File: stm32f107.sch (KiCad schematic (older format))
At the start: 12 parts, among them U5 STM32F107RCTx, Y2 Crystal

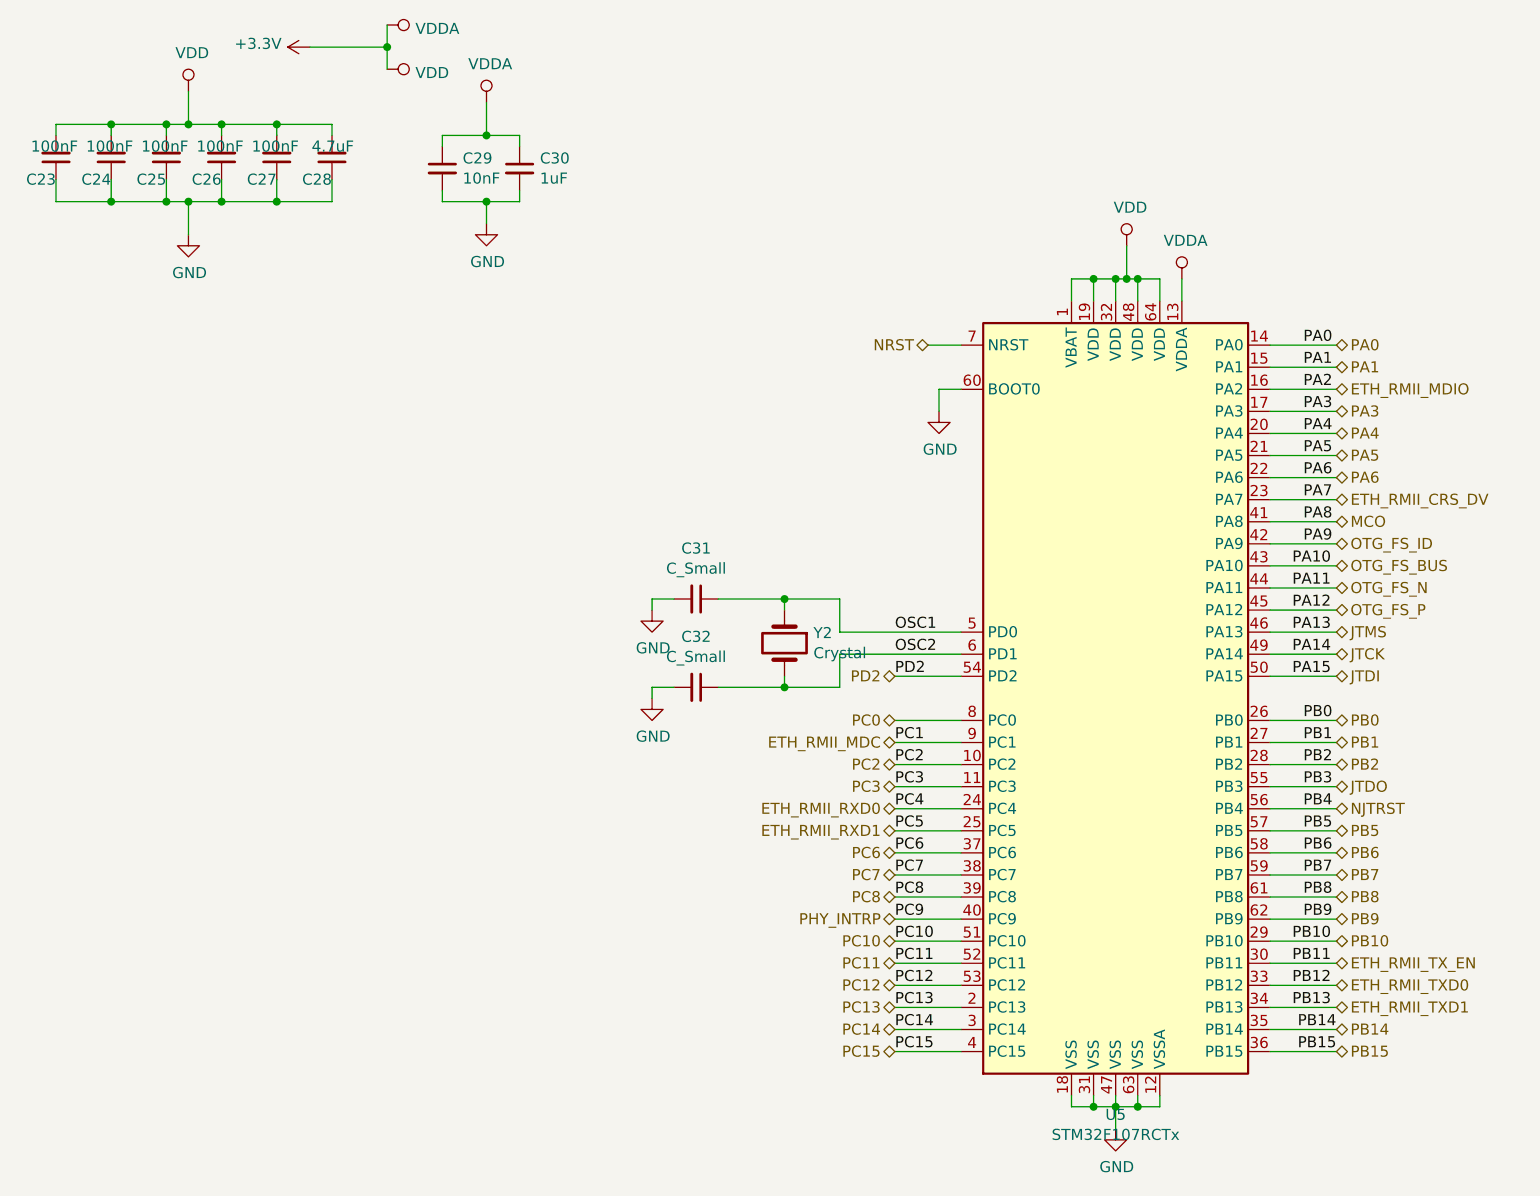
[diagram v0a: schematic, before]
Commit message: pcb updates or something
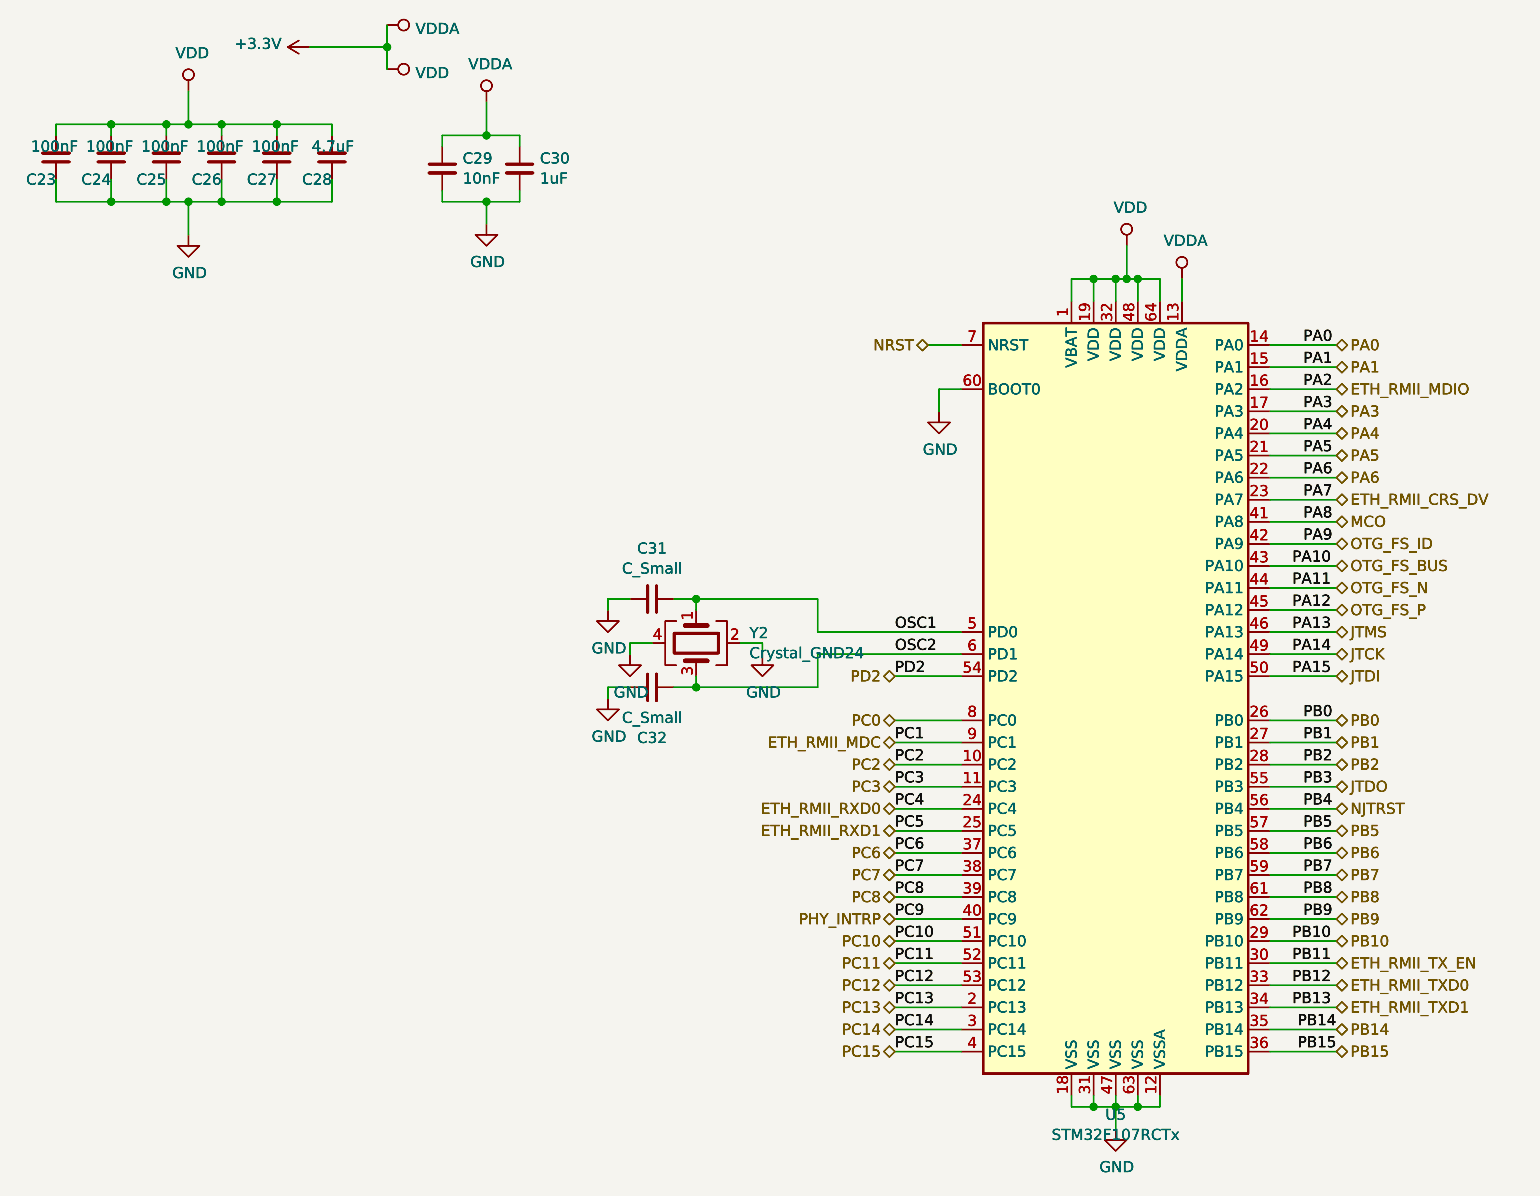
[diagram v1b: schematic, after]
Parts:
- removed Y2: Crystal, symbol Device:Crystal
- added Y2: Crystal_GND24, Crystals:Crystal_SMD_3225-4pin_3.2x2.5mm, symbol Device:Crystal_GND24
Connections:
- net GND: now also C32.1, Y2.2, Y2.4; no longer C32.2
- net OSC1: now also Y2.1
- net OSC2: now also C32.2, Y2.3; no longer C32.1
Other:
- moved on the sheet: C31, C32
